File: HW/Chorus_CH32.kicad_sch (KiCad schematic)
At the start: 19 parts, among them J1 DC_Jack, U1 CH32V003JxMx, U2 TSR_1-2450, U3 TL072

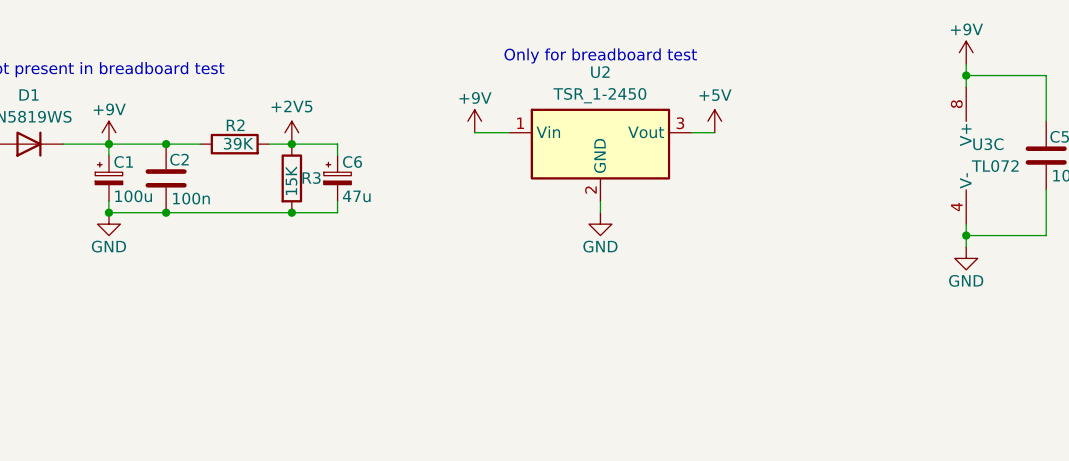
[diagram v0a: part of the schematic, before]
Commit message: d
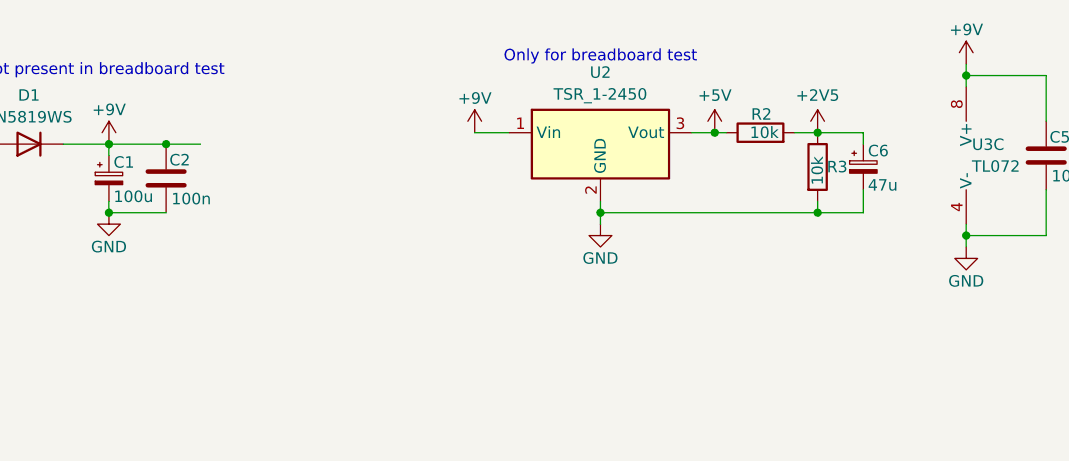
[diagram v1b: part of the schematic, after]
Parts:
- R2: value 39K -> 10k
- R3: value 15K -> 10k
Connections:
- net +5V: now also R2.1
- net +9V: no longer R2.1
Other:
- moved on the sheet: C6, R2, R3
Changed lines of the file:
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@@
 	)
 	(junction
-		(at 78.74 29.21)
+		(at 137.16 27.94)
+		(diameter 0)
+		(color 0 0 0 0)
+	)
+	(junction
+		(at 113.03 36.83)
 		(diameter 0)
 		(color 0 0 0 0)
@@
 	)
 	(junction
-		(at 64.77 36.83)
+		(at 137.16 36.83)
 		(diameter 0)
 		(color 0 0 0 0)
@@
 	)
 	(junction
-		(at 78.74 36.83)
+		(at 58.42 36.83)
 		(diameter 0)
 		(color 0 0 0 0)
 	)
 	(junction
-		(at 58.42 36.83)
+		(at 125.73 27.94)
 		(diameter 0)
 		(color 0 0 0 0)
@@
 	(wire
 		(pts
+			(xy 113.03 38.1) (xy 113.03 36.83)
+		)
+		(stroke
+			(width 0)
+			(type default)
+		)
+	)
+	(wire
+		(pts
 			(xy 30.48 54.61) (xy 33.02 54.61)
 		)
@@
 	(wire
 		(pts
+			(xy 113.03 36.83) (xy 137.16 36.83)
+		)
+		(stroke
+			(width 0)
+			(type default)
+		)
+	)
+	(wire
+		(pts
 			(xy 58.42 36.83) (xy 64.77 36.83)
 		)
@@
 	(wire
 		(pts
-			(xy 78.74 36.83) (xy 83.82 36.83)
+			(xy 137.16 36.83) (xy 142.24 36.83)
 		)
 		(stroke
@@
 	(wire
 		(pts
-			(xy 78.74 29.21) (xy 83.82 29.21)
+			(xy 137.16 27.94) (xy 142.24 27.94)
 		)
 		(stroke
@@
 	(wire
 		(pts
-			(xy 33.02 66.04) (xy 33.02 67.31)
+			(xy 137.16 36.83) (xy 137.16 35.56)
 		)
 		(stroke
@@
 	(wire
 		(pts
-			(xy 40.64 29.21) (xy 31.75 29.21)
+			(xy 33.02 66.04) (xy 33.02 67.31)
 		)
 		(stroke
@@
 	(wire
 		(pts
-			(xy 25.4 124.46) (xy 25.4 125.73)
+			(xy 40.64 29.21) (xy 31.75 29.21)
 		)
 		(stroke
@@
 	(wire
 		(pts
-			(xy 58.42 30.48) (xy 58.42 29.21)
+			(xy 25.4 124.46) (xy 25.4 125.73)
 		)
 		(stroke
@@
 	(wire
 		(pts
-			(xy 64.77 36.83) (xy 78.74 36.83)
+			(xy 58.42 30.48) (xy 58.42 29.21)
 		)
 		(stroke
@@
 	(wire
 		(pts
-			(xy 76.2 29.21) (xy 78.74 29.21)
+			(xy 134.62 27.94) (xy 137.16 27.94)
 		)
 		(stroke
@@
 	(wire
 		(pts
+			(xy 127 27.94) (xy 125.73 27.94)
+		)
+		(stroke
+			(width 0)
+			(type default)
+		)
+	)
+	(wire
+		(pts
 			(xy 33.02 68.58) (xy 33.02 67.31)
 		)
@@
 	(wire
 		(pts
-			(xy 83.82 30.48) (xy 83.82 29.21)
+			(xy 142.24 29.21) (xy 142.24 27.94)
 		)
 		(stroke
@@
 	(wire
 		(pts
-			(xy 83.82 35.56) (xy 83.82 36.83)
+			(xy 142.24 34.29) (xy 142.24 36.83)
 		)
 		(stroke
@@
 	(symbol
 		(lib_id "power:+2V5")
-		(at 78.74 29.21 0)
+		(at 137.16 27.94 0)
 		(unit 1)
 		(exclude_from_sim no)
@@
 		(fields_autoplaced yes)
 		(property "Reference" "#PWR015"
-			(at 78.74 33.02 0)
+			(at 137.16 31.75 0)
 			(effects
 				(font
@@
 		)
 		(property "Value" "+2V5"
-			(at 78.74 25.0769 0)
+			(at 137.16 23.8069 0)
 			(effects
 				(font
@@
 		)
 		(property "Footprint" ""
-			(at 78.74 29.21 0)
+			(at 137.16 27.94 0)
 			(effects
 				(font
@@
 		)
 		(property "Datasheet" ""
-			(at 78.74 29.21 0)
+			(at 137.16 27.94 0)
 			(effects
 				(font
@@
 		)
 		(property "Description" "Power symbol creates a global label with name \"+2V5\""
-			(at 78.74 29.21 0)
+			(at 137.16 27.94 0)
 			(effects
 				(font
@@
 	(symbol
 		(lib_id "power:GND")
-		(at 113.03 36.83 0)
+		(at 113.03 38.1 0)
 		(unit 1)
 		(exclude_from_sim no)
@@
 		(dnp no)
 		(property "Reference" "#PWR07"
-			(at 113.03 43.18 0)
+			(at 113.03 44.45 0)
 			(effects
 				(font
@@
 		)
 		(property "Value" "GND"
-			(at 113.03 40.64 0)
+			(at 113.03 41.91 0)
 			(effects
 				(font
@@
 		)
 		(property "Footprint" ""
-			(at 113.03 36.83 0)
+			(at 113.03 38.1 0)
 			(effects
 				(font
@@
 		)
 		(property "Datasheet" ""
-			(at 113.03 36.83 0)
+			(at 113.03 38.1 0)
 			(effects
 				(font
@@
 		)
 		(property "Description" ""
-			(at 113.03 36.83 0)
+			(at 113.03 38.1 0)
 			(effects
 				(font
@@
 	(symbol
 		(lib_id "Device:C_Polarized_Small")
-		(at 83.82 33.02 0)
+		(at 142.24 31.75 0)
 		(unit 1)
 		(exclude_from_sim no)
@@
 		(dnp no)
 		(property "Reference" "C6"
-			(at 84.328 31.242 0)
+			(at 142.748 29.972 0)
 			(effects
 				(font
@@
 		)
 		(property "Value" "47u"
-			(at 84.328 35.052 0)
+			(at 142.748 33.782 0)
 			(effects
 				(font
@@
 		)
 		(property "Footprint" "Capacitor_SMD:CP_Elec_6.3x5.4"
-			(at 83.82 33.02 0)
+			(at 142.24 31.75 0)
 			(effects
 				(font
@@
 		)
 		(property "Datasheet" "~"
-			(at 83.82 33.02 0)
+			(at 142.24 31.75 0)
 			(effects
 				(font
@@
 		)
 		(property "Description" ""
-			(at 83.82 33.02 0)
+			(at 142.24 31.75 0)
 			(effects
 				(font
@@
 	(symbol
 		(lib_id "Device:R")
-		(at 72.39 29.21 90)
+		(at 130.81 27.94 90)
 		(unit 1)
 		(exclude_from_sim no)
@@
 		(dnp no)
 		(property "Reference" "R2"
-			(at 73.66 27.178 90)
+			(at 132.08 25.908 90)
 			(effects
 				(font
@@
 			)
 		)
-		(property "Value" "39K"
-			(at 74.422 29.21 90)
+		(property "Value" "10k"
+			(at 132.842 27.94 90)
 			(effects
 				(font
@@
 		)
 		(property "Footprint" ""
-			(at 72.39 30.988 90)
+			(at 130.81 29.718 90)
 			(effects
 				(font
@@
 		)
 		(property "Datasheet" "~"
-			(at 72.39 29.21 0)
+			(at 130.81 27.94 0)
 			(effects
 				(font
@@
 		)
 		(property "Description" "Resistor"
-			(at 72.39 29.21 0)
+			(at 130.81 27.94 0)
 			(effects
 				(font
@@
 	(symbol
 		(lib_id "Device:R")
-		(at 78.74 33.02 0)
+		(at 137.16 31.75 0)
 		(unit 1)
 		(exclude_from_sim no)
@@
 		(dnp no)
 		(property "Reference" "R3"
-			(at 79.756 33.02 0)
+			(at 138.176 31.75 0)
 			(effects
 				(font
@@
 			)
 		)
-		(property "Value" "15K"
-			(at 78.74 35.052 90)
+		(property "Value" "10k"
+			(at 137.16 33.782 90)
 			(effects
 				(font
@@
 		)
 		(property "Footprint" ""
-			(at 76.962 33.02 90)
+			(at 135.382 31.75 90)
 			(effects
 				(font
@@
 		)
 		(property "Datasheet" "~"
-			(at 78.74 33.02 0)
+			(at 137.16 31.75 0)
 			(effects
 				(font
@@
 		)
 		(property "Description" "Resistor"
-			(at 78.74 33.02 0)
+			(at 137.16 31.75 0)
 			(effects
 				(font
